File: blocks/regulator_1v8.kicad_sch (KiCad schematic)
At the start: 3 parts, among them U501 TCR2EF 1.8V

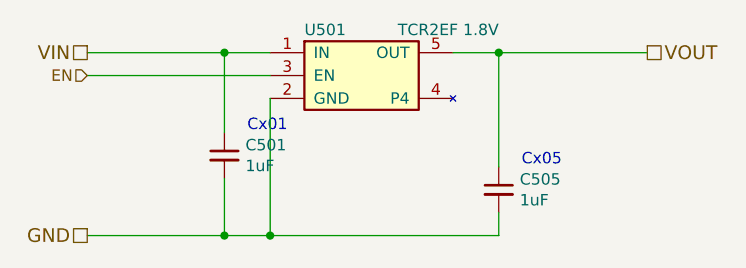
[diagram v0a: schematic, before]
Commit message: Updated references
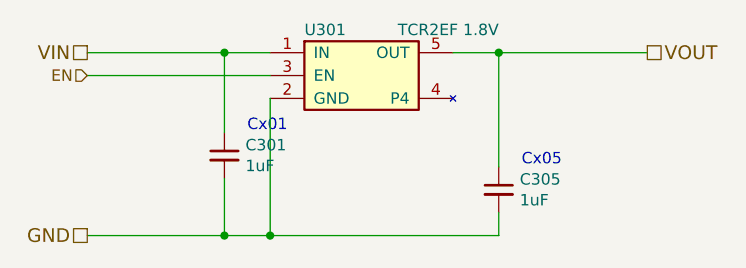
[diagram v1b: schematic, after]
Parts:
- renumbered C501 to C301, C505 to C305, U501 to U301
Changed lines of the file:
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@@
   (symbol (lib_id "Device:C_Small") (at 114.3 105.41 0) (unit 1)
     (in_bom yes) (on_board yes)
-    (property "Reference" "C501" (id 0) (at 116.6368 104.2416 0)
+    (property "Reference" "C301" (id 0) (at 116.6368 104.2416 0)
       (effects (font (size 1.27 1.27)) (justify left))
     )
@@
   (symbol (lib_id "Device:C_Small") (at 144.78 109.22 0) (unit 1)
     (in_bom yes) (on_board yes)
-    (property "Reference" "C505" (id 0) (at 147.1168 108.0516 0)
+    (property "Reference" "C305" (id 0) (at 147.1168 108.0516 0)
       (effects (font (size 1.27 1.27)) (justify left))
     )
@@
   (symbol (lib_id "KwanSystems:ADP122") (at 129.54 96.52 0) (unit 1)
     (in_bom yes) (on_board yes)
-    (property "Reference" "U501" (id 0) (at 123.19 91.44 0)
+    (property "Reference" "U301" (id 0) (at 123.19 91.44 0)
       (effects (font (size 1.27 1.27)) (justify left))
     )

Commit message: updated references
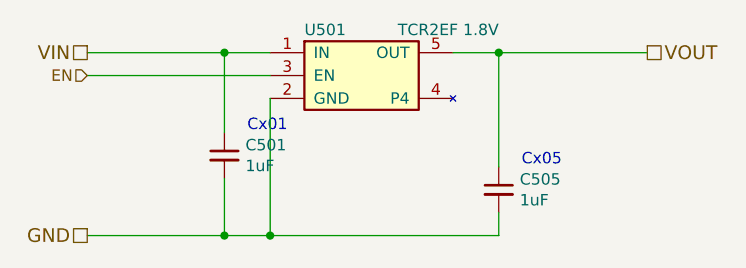
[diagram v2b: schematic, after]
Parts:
- renumbered C301 to C501, C305 to C505, U301 to U501
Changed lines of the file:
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@@
   (symbol (lib_id "Device:C_Small") (at 114.3 105.41 0) (unit 1)
     (in_bom yes) (on_board yes)
-    (property "Reference" "C301" (id 0) (at 116.6368 104.2416 0)
+    (property "Reference" "C501" (id 0) (at 116.6368 104.2416 0)
       (effects (font (size 1.27 1.27)) (justify left))
     )
@@
   (symbol (lib_id "Device:C_Small") (at 144.78 109.22 0) (unit 1)
     (in_bom yes) (on_board yes)
-    (property "Reference" "C305" (id 0) (at 147.1168 108.0516 0)
+    (property "Reference" "C505" (id 0) (at 147.1168 108.0516 0)
       (effects (font (size 1.27 1.27)) (justify left))
     )
@@
   (symbol (lib_id "KwanSystems:ADP122") (at 129.54 96.52 0) (unit 1)
     (in_bom yes) (on_board yes)
-    (property "Reference" "U301" (id 0) (at 123.19 91.44 0)
+    (property "Reference" "U501" (id 0) (at 123.19 91.44 0)
       (effects (font (size 1.27 1.27)) (justify left))
     )
